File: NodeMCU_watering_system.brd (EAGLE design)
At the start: 54.3 x 80 mm, 24 parts, among them IC1 7805DT

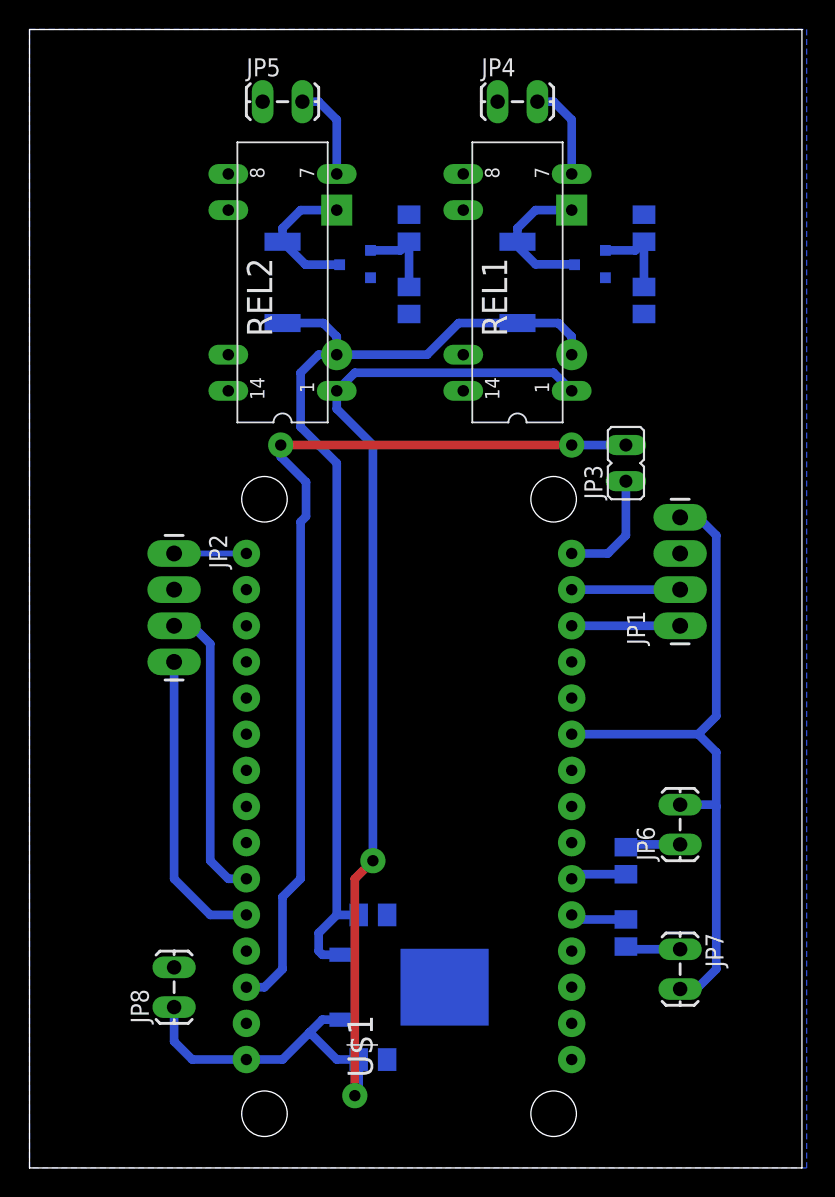
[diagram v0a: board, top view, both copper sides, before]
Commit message: Add files via upload
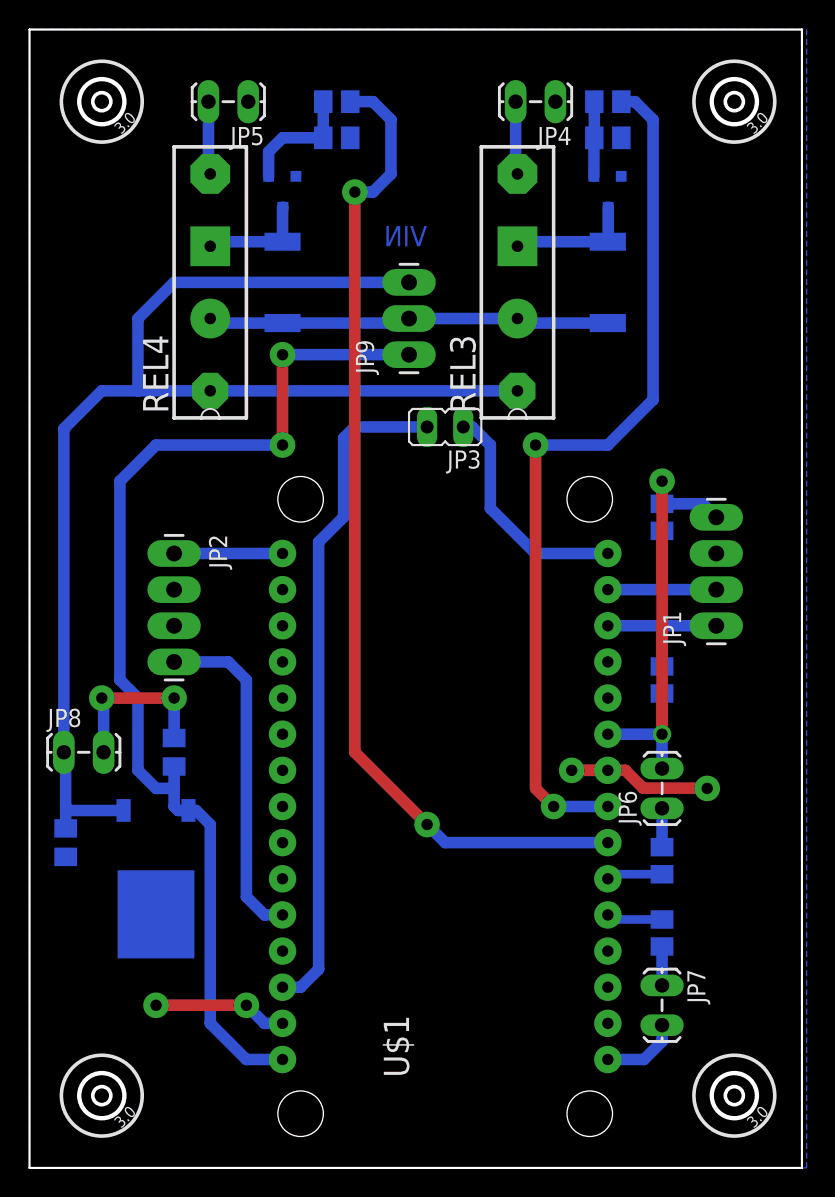
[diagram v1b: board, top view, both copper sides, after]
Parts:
- removed REL1, REL2: RR1A?, #PaJa_22:REL_RR1A
- added JP9: (no value), SparkFun:1X03_LONGPADS
- added R7, R8: 4k7, rcl:M0805
- added REL3, REL4: RELSIA?, #PaJa_22:RELSIA
- added U$2, U$3, U$4, U$5: (no value), #PaJa_30_scr:HOLE_3,0
- C1, C2: value (none) -> 100n
- JP4: value valve -> ouput1
- JP5: value pump -> output2
- JP6: value On/Off -> output1LED
- JP7: value valve on -> ouput2LED
- JP8: value Vin IN -> VIN
- Q1, Q2: value (none) -> IRLML2520
- R1, R3: value 10k -> 1K
- R2, R4: value 10k -> 33K
- R5, R6: value (none) -> 820R
- moved C1 26.4 mm to (2.54, 22.9), turned to 270 degrees
- moved IC1 19.3 mm to (8.89, 20.3), turned to 180 degrees
- moved JP8 19.3 mm to (2.54, 29.2), turned to 0 degrees
- moved C2 18.1 mm to (10.2, 29.2), turned to 90 degrees
- moved R3 14.9 mm to (21.6, 74.9), turned to 0 degrees
- moved R1 14.2 mm to (40.6, 74.9), turned to 0 degrees
- moved JP3 13.0 mm to (29.2, 52.1), turned to 90 degrees
- moved R4 8.13 mm to (21.6, 72.4), turned to 0 degrees
- moved Q2 7.18 mm to (17.8, 68.6), turned to 180 degrees
- moved R2 6.84 mm to (40.6, 72.4), turned to 0 degrees
- moved D1 6.35 mm to (40.6, 62.2)
- moved Q1 5.24 mm to (40.6, 68.6), turned to 180 degrees
- moved JP4 3.81 mm to (36.8, 74.9), turned to 180 degrees
- moved JP7 2.84 mm to (44.5, 12.7)
- moved JP6 2.84 mm to (44.5, 25.4)
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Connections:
- removed net PUMP: R3.1
- removed net VALVE: R1.1
- new net N$10: D1.K, D2.K, JP9.2, REL3.+3, REL4.+3
- new net OUTPUT1: R1.1, U$1.D5
- new net OUTPUT2: R3.1, U$1.D6
- net 3V3: now also R7.2, R8.2, U$1.3V3@2
- net 5V: now also JP9.1, U$1.VIN; no longer D1.K, D2.K, REL1.2, REL2.2
- net GND: now also U$1.GND@1; no longer U$1.GND@0
- net N$4: now also REL3.-5; no longer REL1.6
- net N$5: now also REL4.-5; no longer REL2.6
- net N$6: now also REL3.7; no longer REL1.7
- net N$7: now also REL4.7; no longer REL2.7
- net SCL: now also R7.1
- net SDA: now also R8.1
- net VIN: now also JP9.3, REL3.1, REL4.1; no longer REL1.1, REL2.1, U$1.VIN
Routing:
- net OUTPUT2: track 0.00 -> 70.0 mm, vias 0 -> 2
- net OUTPUT1: track 0.00 -> 62.1 mm, vias 0 -> 2
- net N$10: track 0.00 -> 28.3 mm
- net RST: track 65.6 -> 47.3 mm, vias 2 -> 0
- net GND: track 21.4 -> 33.8 mm, vias 0 -> 6
- net 3V3: track 70.6 -> 62.0 mm, vias 0 -> 2
- net N$1: track 8.15 -> 16.4 mm
- net 5V: track 73.1 -> 77.6 mm, vias 0 -> 2
- net SCL: track 7.62 -> 11.8 mm
- net SDA: track 7.62 -> 10.5 mm
- net AD0: track 5.08 -> 7.62 mm
- net N$3: track 6.14 -> 8.51 mm
- net N$5: track 9.97 -> 7.65 mm
- net N$7: track 6.75 -> 5.13 mm
- net N$6: track 6.75 -> 5.13 mm
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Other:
- board text added: "VIN"
